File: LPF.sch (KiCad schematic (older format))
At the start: 107 parts, among them P1 SMA, P2 J5/J5' Ctrl Brd, P3 SMA, P4 SMA

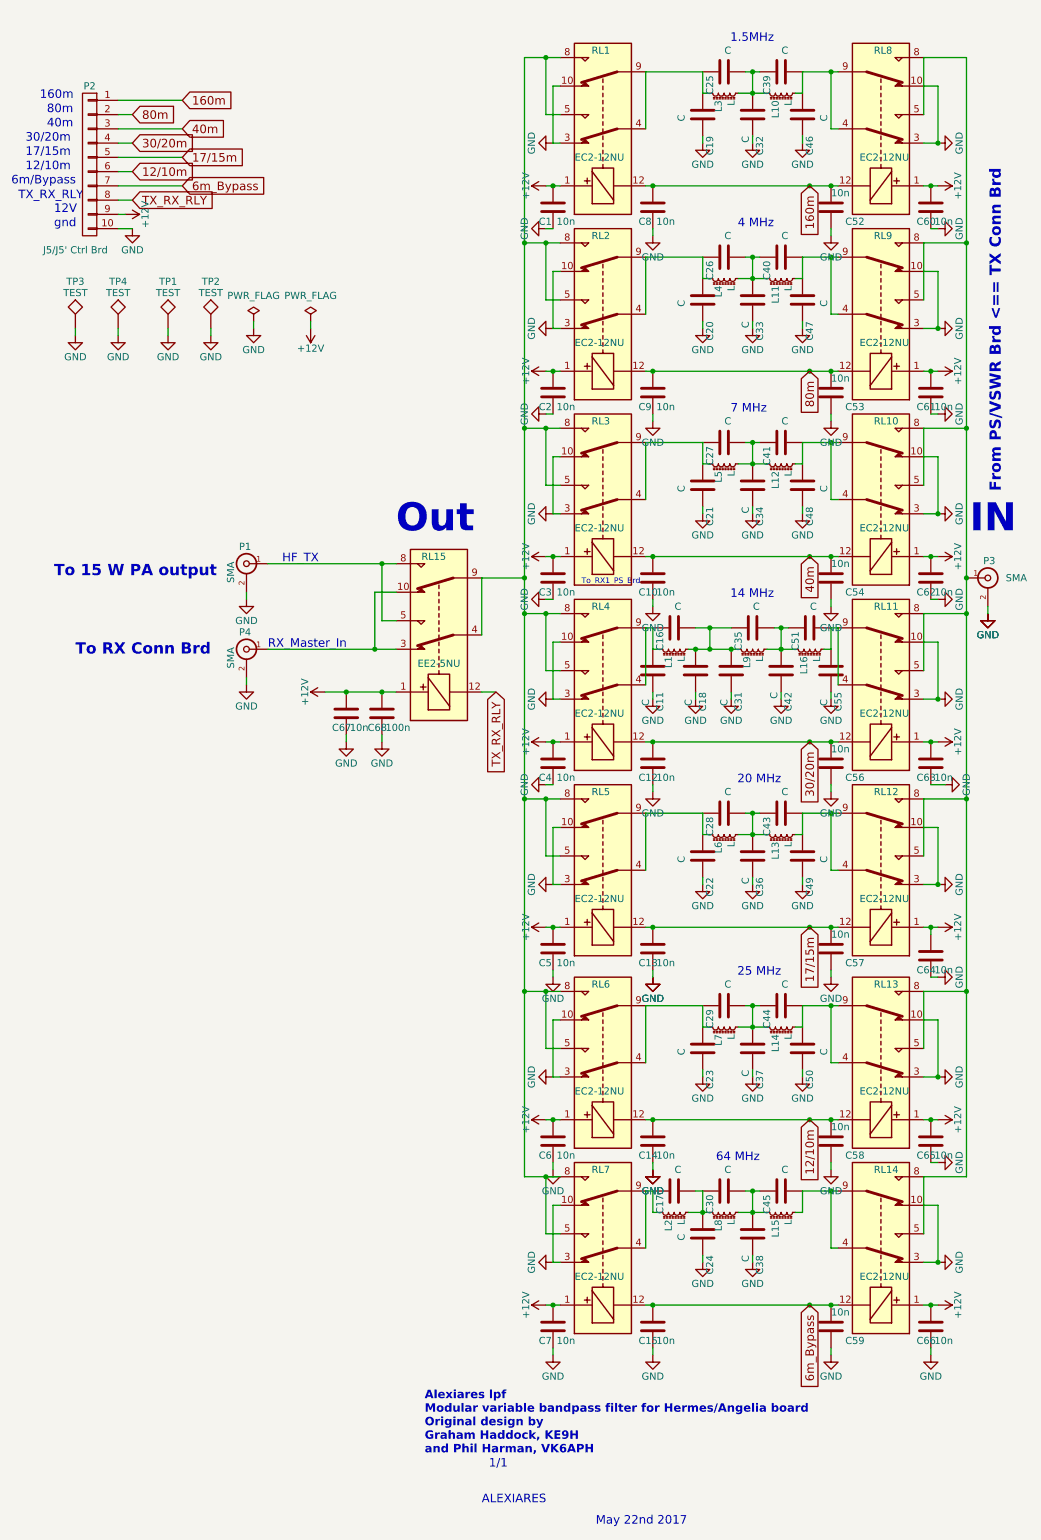
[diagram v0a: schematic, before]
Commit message: version 1.1
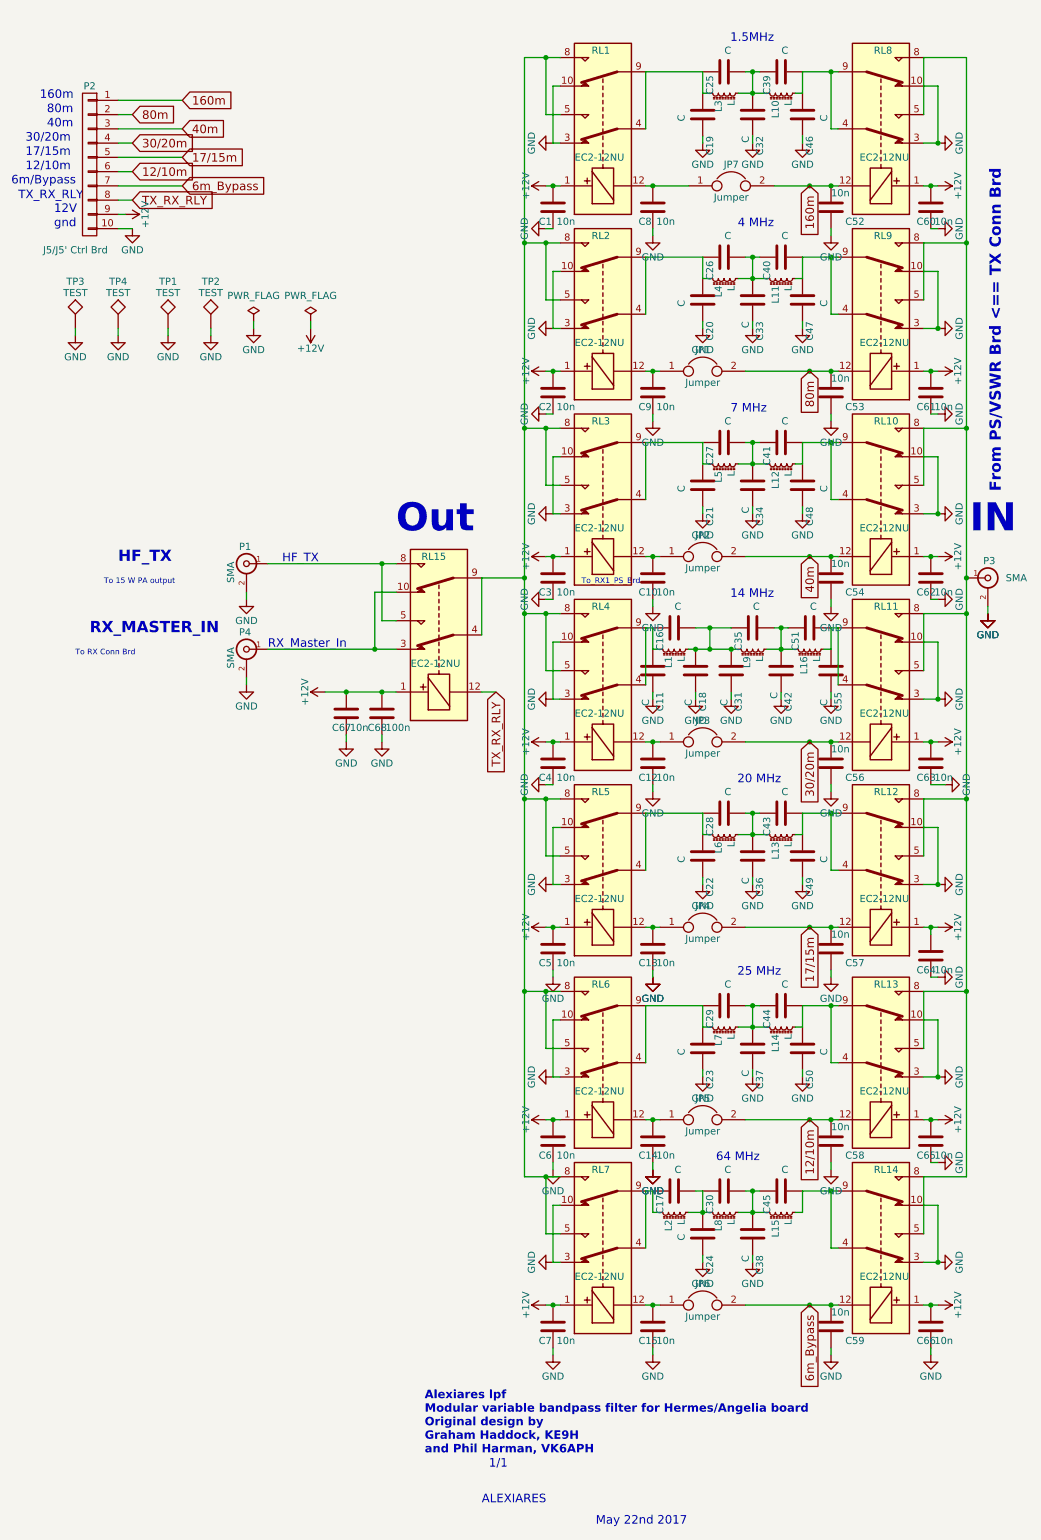
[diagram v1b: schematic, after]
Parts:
- added JP1, JP2, JP3, JP4, JP5, JP6, JP7: Jumper, Jumper:Coax_wire_1.20m_Drill, symbol Jumper
- RL15: value EE2-5NU -> EC2-12NU
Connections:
- net 12/10m: now also JP5.2; no longer C14.1, RL6.12
- net 160m: now also JP7.2; no longer C8.1, RL1.12
- net 17/15m: now also JP4.2; no longer C13.1, RL5.12
- net 30/20m: now also JP3.2; no longer C12.1, RL4.12
- net 40m: now also JP2.2; no longer C10.1, RL3.12
- net 6m_Bypass: now also JP6.2; no longer C15.1, RL7.12
- net 80m: now also JP1.2; no longer C9.1, RL2.12
- new net: C8.1, JP7.1, RL1.12
- new net: C12.1, JP3.1, RL4.12
- new net: C15.1, JP6.1, RL7.12
- new net: C10.1, JP2.1, RL3.12
- new net: C9.1, JP1.1, RL2.12
- new net: C13.1, JP4.1, RL5.12
- new net: C14.1, JP5.1, RL6.12
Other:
- note added: "RX_MASTER_IN"
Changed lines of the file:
@@
 	5200 1950 5200 2000
-Wire Wire Line
-	5150 1650 6500 1650
 Wire Wire Line
 	4450 1650 4550 1650
@@
 	7150 3250 7200 3250
 Wire Wire Line
-	5150 2950 6500 2950
-Wire Wire Line
 	6450 3250 6450 3300
 Wire Wire Line
@@
 	7150 4550 7200 4550
 Wire Wire Line
-	5150 4250 6500 4250
-Wire Wire Line
 	6450 4550 6450 4600
 Wire Wire Line
@@
 	7150 5850 7250 5850
 Wire Wire Line
-	5150 5550 6500 5550
-Wire Wire Line
 	6450 5850 6450 5900
 Wire Wire Line
@@
 	7150 9800 7150 9850
 Wire Wire Line
-	5150 9500 6500 9500
-Wire Wire Line
 	6450 9800 6450 9850
 Wire Wire Line
@@
 	7200 7200 7150 7200
 Wire Wire Line
-	5150 6850 6500 6850
-Wire Wire Line
 	6450 7150 6450 7200
 Wire Wire Line
@@
 Wire Wire Line
 	7150 8500 7200 8500
-Wire Wire Line
-	5150 8200 6500 8200
 Wire Wire Line
 	6450 8500 6450 8550
@@
 P 3700 5000
 F 0 "RL15" V 4450 4950 50  0000 L CNN
-F 1 "EE2-5NU" V 3700 4850 50  0000 L CNN
+F 1 "EC2-12NU" V 3700 4850 50  0000 L CNN
 F 2 "2_Form_C_Relay:THT_2_formC" H 3700 5000 50  0001 C CNN
 F 3 "" H 3700 5000 50  0001 C CNN
@@
 Text GLabel 4100 5200 3    60   Input ~ 0
 TX_RX_RLY
-Text Notes 1150 4950 0    79   ~ 16
+Text Notes 1150 4950 0    39   ~ 0
 To RX Conn Brd\n
-Text Notes 1000 4400 0    79   ~ 16
+Text Notes 1350 4450 0    39   ~ 0
 To 15 W PA output\n
 Text Notes 7650 3800 1    79   ~ 16
@@
 Wire Wire Line
 	2800 2600 2800 2650
+Text Notes 1250 4800 0    79   ~ 16
+RX_MASTER_IN
+Text Notes 1450 4300 0    79   ~ 16
+HF_TX
+$Comp
+L Jumper JP1
+U 1 1 5946D769
+P 5550 2950
+F 0 "JP1" H 5550 3100 50  0000 C CNN
+F 1 "Jumper" H 5550 2870 50  0000 C CNN
+F 2 "Jumper:Coax_wire_1.20m_Drill" H 5550 2950 50  0001 C CNN
+F 3 "" H 5550 2950 50  0001 C CNN
+	1    5550 2950
+	1    0    0    -1
+$EndComp
+$Comp
+L Jumper JP7
+U 1 1 5946F7F4
+P 5750 1650
+F 0 "JP7" H 5750 1800 50  0000 C CNN
+F 1 "Jumper" H 5750 1570 50  0000 C CNN
+F 2 "Jumper:Coax_wire_1.20m_Drill" H 5750 1650 50  0001 C CNN
+F 3 "" H 5750 1650 50  0001 C CNN
+	1    5750 1650
+	1    0    0    -1
+$EndComp
+Wire Wire Line
+	5150 1650 5450 1650
+Wire Wire Line
+	6050 1650 6500 1650
+$Comp
+L Jumper JP2
+U 1 1 59472F9F
+P 5550 4250
+F 0 "JP2" H 5550 4400 50  0000 C CNN
+F 1 "Jumper" H 5550 4170 50  0000 C CNN
+F 2 "Jumper:Coax_wire_1.20m_Drill" H 5550 4250 50  0001 C CNN
+F 3 "" H 5550 4250 50  0001 C CNN
+	1    5550 4250
+	1    0    0    -1
+$EndComp
+$Comp
+L Jumper JP3
+U 1 1 59473567
+P 5550 5550
+F 0 "JP3" H 5550 5700 50  0000 C CNN
+F 1 "Jumper" H 5550 5470 50  0000 C CNN
+F 2 "Jumper:Coax_wire_1.20m_Drill" H 5550 5550 50  0001 C CNN
+F 3 "" H 5550 5550 50  0001 C CNN
+	1    5550 5550
+	1    0    0    -1
+$EndComp
+$Comp
+L Jumper JP4
+U 1 1 5947360C
+P 5550 6850
+F 0 "JP4" H 5550 7000 50  0000 C CNN
+F 1 "Jumper" H 5550 6770 50  0000 C CNN
+F 2 "Jumper:Coax_wire_1.20m_Drill" H 5550 6850 50  0001 C CNN
+F 3 "" H 5550 6850 50  0001 C CNN
+	1    5550 6850
+	1    0    0    -1
+$EndComp
+$Comp
+L Jumper JP5
+U 1 1 59473A3C
+P 5550 8200
+F 0 "JP5" H 5550 8350 50  0000 C CNN
+F 1 "Jumper" H 5550 8120 50  0000 C CNN
+F 2 "Jumper:Coax_wire_1.20m_Drill" H 5550 8200 50  0001 C CNN
+F 3 "" H 5550 8200 50  0001 C CNN
+	1    5550 8200
+	1    0    0    -1
+$EndComp
+$Comp
+L Jumper JP6
+U 1 1 59473AE3
+P 5550 9500
+F 0 "JP6" H 5550 9650 50  0000 C CNN
+F 1 "Jumper" H 5550 9420 50  0000 C CNN
+F 2 "Jumper:Coax_wire_1.20m_Drill" H 5550 9500 50  0001 C CNN
+F 3 "" H 5550 9500 50  0001 C CNN
+	1    5550 9500
+	1    0    0    -1
+$EndComp
+Wire Wire Line
+	5150 6850 5250 6850
+Wire Wire Line
+	5850 6850 6500 6850
+Wire Wire Line
+	5150 9500 5250 9500
+Wire Wire Line
+	5850 9500 6500 9500
+Wire Wire Line
+	5850 8200 6500 8200
+Wire Wire Line
+	5150 8200 5250 8200
+Wire Wire Line
+	5150 5550 5250 5550
+Wire Wire Line
+	5850 5550 6500 5550
+Wire Wire Line
+	5150 4250 5250 4250
+Wire Wire Line
+	5850 4250 6500 4250
+Wire Wire Line
+	5150 2950 5250 2950
+Wire Wire Line
+	5850 2950 6500 2950
 $EndSCHEMATC

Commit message: minor changes, adding kk lib, still under dev.
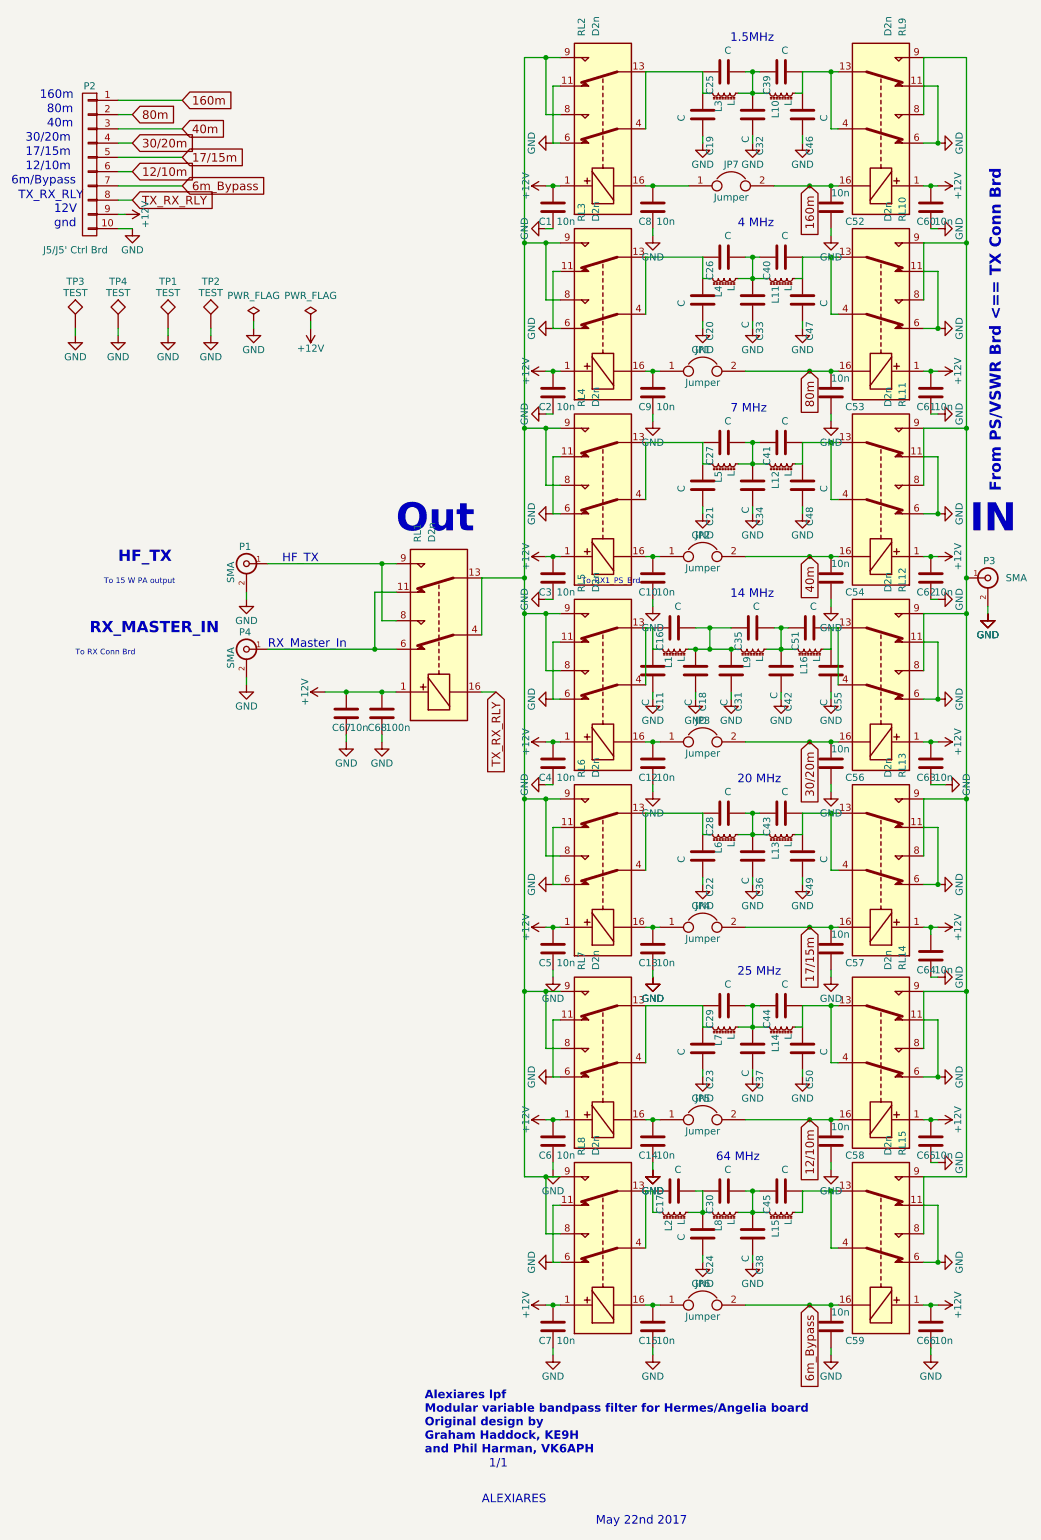
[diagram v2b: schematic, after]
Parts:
- removed RL1, RL10, RL11, RL12, RL13, RL14, RL15, RL2, RL3, RL4, RL5, RL6, RL7, RL8, RL9: EC2-12NU, 2_Form_C_Relay:THT_2_formC, symbol EE2-5NU
- added RL1, RL10, RL11, RL12, RL13, RL14, RL15, RL2, RL3, RL4, RL5, RL6, RL7, RL8, RL9: D2n, symbol D2n
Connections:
- net +12V: now also RL1.1, RL10.1, RL11.1, RL12.1, RL13.1, RL14.1, RL15.1, RL2.1, RL3.1, RL4.1, RL5.1, RL6.1, RL7.1, RL8.1, RL9.1
- net 12/10m: now also RL14.16
- net 160m: now also RL9.16
- net 17/15m: now also RL13.16
- net 30/20m: now also RL12.16
- net 40m: now also RL11.16
- net 6m_Bypass: now also RL15.16
- net 80m: now also RL10.16
- net GND: now also RL10.11, RL10.6, RL11.11, RL11.6, RL12.11, RL12.6, RL13.11, RL13.6, RL14.11, RL14.6, RL15.11, RL15.6, RL2.11, RL2.6, RL3.11, RL3.6, RL4.11, RL4.6, RL5.11, RL5.6, RL6.11, RL6.6, RL7.11, RL7.6, RL8.11, RL8.6, RL9.11, RL9.6
- net TX_RX_RLY: now also RL1.16
- net at P3.1 (In): now also RL10.8, RL10.9, RL11.8, RL11.9, RL12.8, RL12.9, RL13.8, RL13.9, RL14.8, RL14.9, RL15.8, RL15.9, RL9.8, RL9.9
- net at C8.1, JP7.1: now also RL2.16
- net at C19.2, C25.1, L3.1: now also RL2.13, RL2.4
- net at C39.2, C46.2, L10.2: now also RL9.13, RL9.4
- net at C40.2, C47.2, L11.2: now also RL10.13, RL10.4
- net at C20.2, C26.1, L4.1: now also RL3.13, RL3.4
- net at C41.2, C48.2, L12.2: now also RL11.13, RL11.4
- net at C21.2, C27.1, L5.1: now also RL4.13, RL4.4
- net at C51.2, C55.2, L16.2: now also RL12.13, RL12.4
- net at C45.2, L15.2: now also RL15.13, RL15.4
- net at C43.2, C49.2, L13.2: now also RL13.13, RL13.4
- net at C22.2, C28.1, L6.1: now also RL6.13, RL6.4
- net at C44.2, C50.2, L14.2: now also RL14.13, RL14.4
- net at C23.2, C29.1, L7.1: now also RL7.13, RL7.4
- net at C17.1, L2.1: now also RL8.13, RL8.4
- net at C11.2, C16.1, L1.1: now also RL5.13, RL5.4
- net at C12.1, JP3.1: now also RL5.16
- net at C15.1, JP6.1: now also RL8.16
- net at C10.1, JP2.1: now also RL4.16
- net at C9.1, JP1.1: now also RL3.16
- net at C13.1, JP4.1: now also RL6.16
- net at C14.1, JP5.1: now also RL7.16
- net at P1.1 (In): now also RL1.8, RL1.9
- net at P4.1 (In): now also RL1.11, RL1.6
- new net: RL1.13, RL1.4, RL2.8, RL2.9, RL3.8, RL3.9, RL4.8, RL4.9, RL5.8, RL5.9, RL6.8, RL6.9, RL7.8, RL7.9, RL8.8, RL8.9
